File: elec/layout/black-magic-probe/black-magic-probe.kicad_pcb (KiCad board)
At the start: 2 copper layers, 48.1 x 19.2 mm, 61 parts

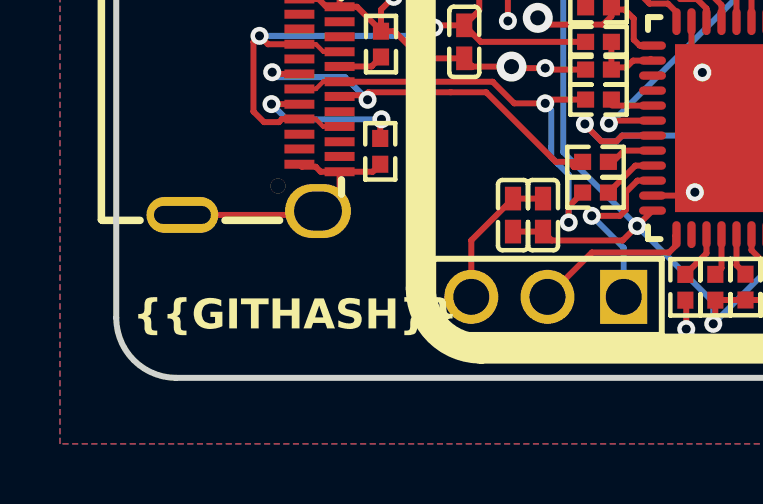
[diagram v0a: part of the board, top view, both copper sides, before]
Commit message: checkin
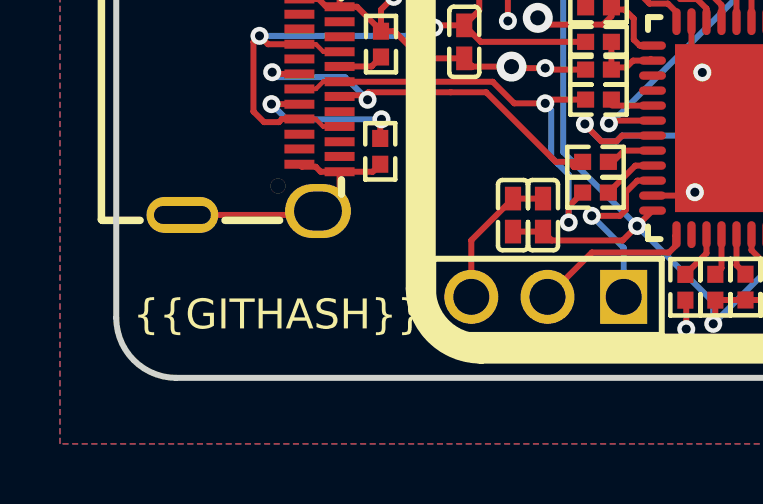
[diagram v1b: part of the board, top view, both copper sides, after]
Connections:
- net CC1 renamed A5
- net G2 renamed black_magic_debugger-G2-1
- net black_magic_debugger-G1 renamed black_magic_debugger-G2
- C1 pad 1: hv-1 -> hv
- C10 pad 1: hv-1 -> hv
- C11 pad 1: hv-1 -> hv
- C15 pad 1: black_magic_debugger-line -> black_magic_debugger-line-3
- C17 pad 1: hv-1 -> hv
- C2 pad 1: hv-1 -> hv
- C3 pad 1: hv-1 -> hv
- C4 pad 1: hv-1 -> hv
- C5 pad 1: hv-1 -> hv
- C6 pad 1: hv-1 -> hv
- C7 pad 1: hv-1 -> hv
- C8 pad 1: hv-1 -> hv
- C9 pad 1: hv-1 -> hv
- D2 pad 1: black_magic_debugger-anode-1 -> black_magic_debugger-anode
- D3 pad 1: black_magic_debugger-anode -> black_magic_debugger-anode-1
- R1 pad 2: hv-1 -> hv
- R10 pad 1: line-4 -> line-3
- R11 pad 2: hv-1 -> hv
- R14 pad 2: line-1 -> line-4
- R15 pad 1: black_magic_debugger-B2-1 -> black_magic_debugger-B2-3
- R15 pad 2: line-5 -> line-2
- R16 pad 2: line-2 -> line-1
- R17 pad 1: black_magic_debugger-B2 -> black_magic_debugger-B2-2
- R18 pad 2: line-2 -> line-1
- R19 pad 1: black_magic_debugger-B2-3 -> black_magic_debugger-B2-1
- R19 pad 2: black_magic_debugger-line-4 -> black_magic_debugger-line-5
- R2 pad 2: hv-1 -> hv
- R20 pad 1: black_magic_debugger-B2-2 -> black_magic_debugger-B2
- R20 pad 2: black_magic_debugger-line-7 -> black_magic_debugger-line-8
- R21 pad 1: black_magic_debugger-line-2 -> black_magic_debugger-line
- R22 pad 2: black_magic_debugger-line-2 -> black_magic_debugger-line
- R23 pad 1: black_magic_debugger-line -> black_magic_debugger-line-3
- R24 pad 1: hv -> hv-1
- R24 pad 2: black_magic_debugger-line -> black_magic_debugger-line-3
- R25 pad 2: hv -> hv-1
- R27 pad 1: hv-1 -> hv
- R3 pad 2: hv-1 -> hv
- R8 pad 1: line-4 -> line-3
- R9 pad 1: line-3 -> line-5
- U1 pad 1: hv-1 -> hv
- U1 pad 5: hv-1 -> hv
- U1 pad 6: black_magic_debugger-B2-2 -> black_magic_debugger-B2
- U2 pad 1: hv-1 -> hv
- U2 pad 2: black_magic_debugger-line-8 -> black_magic_debugger-line-7
- U2 pad 3: black_magic_debugger-line-5 -> black_magic_debugger-line-4
- U2 pad 5: hv-1 -> hv
- U2 pad 6: black_magic_debugger-B2-1 -> black_magic_debugger-B2-3
- U3 pad 1: hv-1 -> hv
- U3 pad 2: black_magic_debugger-line-6 -> black_magic_debugger-line-2
- U3 pad 3: black_magic_debugger-line-3 -> black_magic_debugger-line-1
- U3 pad 6: black_magic_debugger-B2-3 -> black_magic_debugger-B2-1
- U4 pad 1: hv-1 -> hv
- U4 pad 3: black_magic_debugger-line-1 -> black_magic_debugger-line-6
- U4 pad 6: black_magic_debugger-B2 -> black_magic_debugger-B2-2
- U5 pad 1: hv-1 -> hv
- U5 pad 13: black_magic_debugger-line-5 -> black_magic_debugger-line-4
- U5 pad 14: black_magic_debugger-line-1 -> black_magic_debugger-line-6
- U5 pad 15: black_magic_debugger-line-8 -> black_magic_debugger-line-7
- U5 pad 16: black_magic_debugger-line-6 -> black_magic_debugger-line-2
- U5 pad 18: black_magic_debugger-line -> black_magic_debugger-line-3
- U5 pad 21: black_magic_debugger-anode-1 -> black_magic_debugger-anode
- U5 pad 22: black_magic_debugger-anode -> black_magic_debugger-anode-1
- U5 pad 24: hv-1 -> hv
- U5 pad 26: black_magic_debugger-line-2 -> black_magic_debugger-line
- U5 pad 31: black_magic_debugger-line-3 -> black_magic_debugger-line-1
- U5 pad 36: hv-1 -> hv
- U5 pad 48: hv-1 -> hv
- U5 pad 9: hv-1 -> hv
- U6 pad 3: hv -> hv-1
- U6 pad 6: hv-1 -> hv
- U7 pad 4: hv-1 -> hv
- U8 pad 1: hv -> hv-1
- U8 pad 4: line-1 -> line-4
- U8 pad 6: line-2 -> line-1
- U8 pad 8: line-5 -> line-2
- U9 pad 5: hv-1 -> hv
- USB1 pad A6: line-4 -> line-3
- USB1 pad A7: line-3 -> line-5
- USB1 pad B6: line-4 -> line-3
- USB1 pad B7: line-3 -> line-5
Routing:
- net hv-1: track 121.3 -> 36.1 mm, vias 11 -> 2
- net hv: track 36.1 -> 121.3 mm, vias 2 -> 11
- net line-2: track 28.0 -> 4.28 mm, vias 2 -> 0
- net line-1: track 6.64 -> 28.0 mm
- net black_magic_debugger-line-2: track 2.58 -> 17.1 mm
- net black_magic_debugger-line-8: track 14.1 -> 0.00 mm, vias 2 -> 0
- net black_magic_debugger-line-7: track 0.00 -> 14.1 mm, vias 0 -> 2
- net black_magic_debugger-line-3: track 20.3 -> 7.33 mm, vias 2 -> 0
- net black_magic_debugger-line-5: track 10.8 -> 0.00 mm, vias 2 -> 0
- net black_magic_debugger-line-4: track 0.00 -> 10.8 mm, vias 0 -> 2
- net line-5: track 4.28 -> 14.8 mm, vias 0 -> 2
- net line-4: track 15.5 -> 6.64 mm
- net black_magic_debugger-line: track 7.33 -> 2.58 mm
- net black_magic_debugger-line-1: track 16.8 -> 20.3 mm
- net line-3: track 14.8 -> 15.5 mm
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
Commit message: build with excluded checks
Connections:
- net A5 renamed CC1
- net CC2 renamed B5
- net S2 renamed S1
- C1 pad 1: hv -> hv-2
- C10 pad 1: hv -> hv-2
- C11 pad 1: hv -> hv-2
- C15 pad 1: black_magic_debugger-line-3 -> black_magic_debugger-line-2
- C16 pad 1: hv-2 -> hv
- C17 pad 1: hv -> hv-2
- C2 pad 1: hv -> hv-2
- C3 pad 1: hv -> hv-2
- C4 pad 1: hv -> hv-2
- C5 pad 1: hv -> hv-2
- C6 pad 1: hv -> hv-2
- C7 pad 1: hv -> hv-2
- C8 pad 1: hv -> hv-2
- C9 pad 1: hv -> hv-2
- D1 pad 1: black_magic_debugger-anode-2 -> black_magic_debugger-anode
- D2 pad 1: black_magic_debugger-anode -> black_magic_debugger-anode-2
- R1 pad 2: hv -> hv-2
- R10 pad 1: line-3 -> line-5
- R11 pad 2: hv -> hv-2
- R12 pad 1: black_magic_debugger-G2 -> black_magic_debugger-G2-1
- R14 pad 2: line-4 -> line-3
- R15 pad 1: black_magic_debugger-B2-3 -> black_magic_debugger-B2-2
- R15 pad 2: line-2 -> line-4
- R16 pad 2: line-1 -> line-2
- R17 pad 1: black_magic_debugger-B2-2 -> black_magic_debugger-B2-1
- R18 pad 2: line-1 -> line-2
- R19 pad 1: black_magic_debugger-B2-1 -> black_magic_debugger-B2-3
- R19 pad 2: black_magic_debugger-line-5 -> black_magic_debugger-line-6
- R2 pad 2: hv -> hv-2
- R20 pad 2: black_magic_debugger-line-8 -> black_magic_debugger-line-7
- R21 pad 1: black_magic_debugger-line -> black_magic_debugger-line-5
- R22 pad 1: hv-2 -> hv
- R22 pad 2: black_magic_debugger-line -> black_magic_debugger-line-5
- R23 pad 1: black_magic_debugger-line-3 -> black_magic_debugger-line-2
- R24 pad 2: black_magic_debugger-line-3 -> black_magic_debugger-line-2
- R27 pad 1: hv -> hv-2
- R3 pad 2: hv -> hv-2
- R8 pad 1: line-3 -> line-5
- R9 pad 1: line-5 -> line-1
- U1 pad 1: hv -> hv-2
- U1 pad 3: black_magic_debugger-line-9 -> black_magic_debugger-line-4
- U1 pad 5: hv -> hv-2
- U2 pad 1: hv -> hv-2
- U2 pad 2: black_magic_debugger-line-7 -> black_magic_debugger-line-1
- U2 pad 3: black_magic_debugger-line-4 -> black_magic_debugger-line
- U2 pad 5: hv -> hv-2
- U2 pad 6: black_magic_debugger-B2-3 -> black_magic_debugger-B2-2
- U3 pad 1: hv -> hv-2
- U3 pad 2: black_magic_debugger-line-2 -> black_magic_debugger-line-3
- U3 pad 3: black_magic_debugger-line-1 -> black_magic_debugger-line-8
- U3 pad 6: black_magic_debugger-B2-1 -> black_magic_debugger-B2-3
- U4 pad 1: hv -> hv-2
- U4 pad 3: black_magic_debugger-line-6 -> black_magic_debugger-line-9
- U4 pad 6: black_magic_debugger-B2-2 -> black_magic_debugger-B2-1
- U5 pad 1: hv -> hv-2
- U5 pad 12: black_magic_debugger-G2-1 -> black_magic_debugger-G2
- U5 pad 13: black_magic_debugger-line-4 -> black_magic_debugger-line
- U5 pad 14: black_magic_debugger-line-6 -> black_magic_debugger-line-9
- U5 pad 15: black_magic_debugger-line-7 -> black_magic_debugger-line-1
- U5 pad 16: black_magic_debugger-line-2 -> black_magic_debugger-line-3
- U5 pad 18: black_magic_debugger-line-3 -> black_magic_debugger-line-2
- U5 pad 19: black_magic_debugger-G2 -> black_magic_debugger-G2-1
- U5 pad 20: black_magic_debugger-anode-2 -> black_magic_debugger-anode
- U5 pad 21: black_magic_debugger-anode -> black_magic_debugger-anode-2
- U5 pad 24: hv -> hv-2
- U5 pad 26: black_magic_debugger-line -> black_magic_debugger-line-5
- U5 pad 30: black_magic_debugger-line-9 -> black_magic_debugger-line-4
- U5 pad 31: black_magic_debugger-line-1 -> black_magic_debugger-line-8
- U5 pad 36: hv -> hv-2
- U5 pad 48: hv -> hv-2
- U5 pad 9: hv -> hv-2
- U6 pad 2: black_magic_debugger-G2 -> black_magic_debugger-G2-1
- U6 pad 5: black_magic_debugger-G2 -> black_magic_debugger-G2-1
- U6 pad 6: hv -> hv-2
- U7 pad 2: black_magic_debugger-G2-1 -> black_magic_debugger-G2
- U7 pad 4: hv -> hv-2
- U8 pad 4: line-4 -> line-3
- U8 pad 6: line-1 -> line-2
- U8 pad 8: line-2 -> line-4
- U9 pad 1: hv-2 -> hv
- U9 pad 3: hv-2 -> hv
- U9 pad 5: hv -> hv-2
- USB1 pad A4: hv-2 -> hv
- USB1 pad A6: line-3 -> line-5
- USB1 pad A7: line-5 -> line-1
- USB1 pad A9: hv-2 -> hv
- USB1 pad B4: hv-2 -> hv
- USB1 pad B6: line-3 -> line-5
- USB1 pad B7: line-5 -> line-1
- USB1 pad B9: hv-2 -> hv
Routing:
- net hv-2: track 25.5 -> 121.3 mm, vias 2 -> 11
- net hv: track 121.3 -> 25.5 mm, vias 11 -> 2
- net line-2: track 4.28 -> 28.0 mm, vias 0 -> 2
- net black_magic_debugger-line-8: track 0.00 -> 20.3 mm, vias 0 -> 2
- net black_magic_debugger-line-6: track 16.8 -> 0.00 mm, vias 2 -> 0
- net black_magic_debugger-line-7: track 14.1 -> 0.00 mm, vias 2 -> 0
- net line-1: track 28.0 -> 14.8 mm
- net black_magic_debugger-line-4: track 10.8 -> 22.8 mm
- net black_magic_debugger-line-3: track 7.33 -> 17.1 mm
- net black_magic_debugger-line-2: track 17.1 -> 7.33 mm
- net line-3: track 15.5 -> 6.64 mm
- net black_magic_debugger-line: track 2.58 -> 10.8 mm, vias 0 -> 2
- net black_magic_debugger-line-1: track 20.3 -> 14.1 mm
- net black_magic_debugger-line-9: track 22.8 -> 16.8 mm
- net black_magic_debugger-G2-1: track 12.1 -> 7.11 mm, vias 2 -> 0
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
